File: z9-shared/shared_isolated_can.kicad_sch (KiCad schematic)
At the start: 6 parts, among them U951 ISO1042-Q1

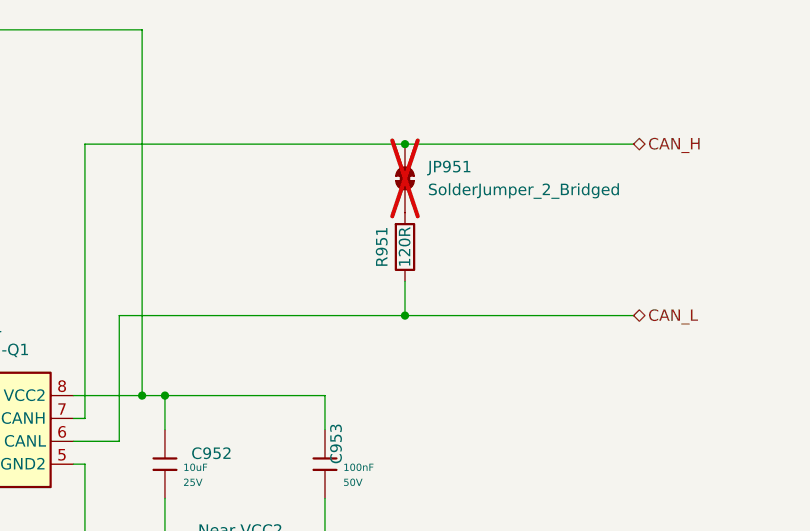
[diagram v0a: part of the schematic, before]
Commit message: lcsc components and cleanup
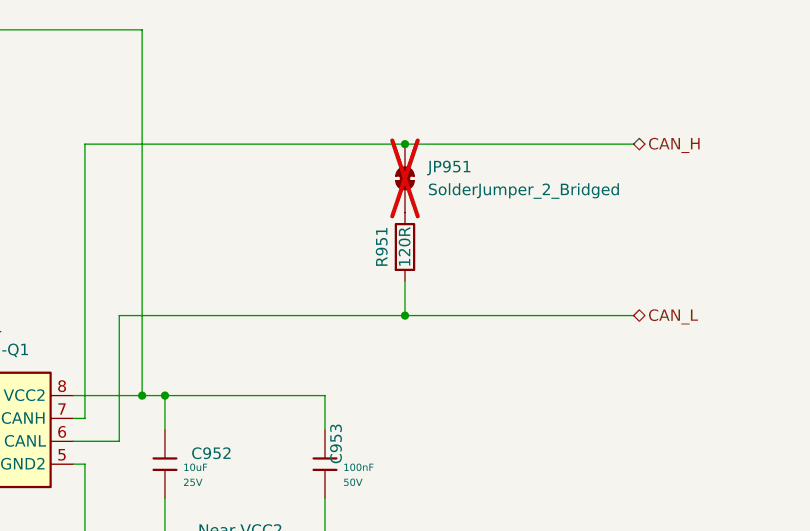
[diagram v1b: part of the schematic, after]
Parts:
- R951: footprint Resistor_SMD:R_0805_2012Metric -> dnt:R_1206_3216Metric; symbol dnt_global:Resisitor_120R_0805 -> dnt_global:Resistor_-_1206,120Ω; Attrition Qty (none) -> 10; Category (none) -> Resistors,Chip Resistor - Surface Mount; Class (none) -> Basic Component; LCSC (none) -> C17909; Manufacturer (none) -> UNI-ROYAL(Uniroyal Elec); Minimum Qty (none) -> 15; Operating Temperature Range (none) -> -55°C~+155°C; Overload Voltage (Max) (none) -> 200V; Part (none) -> 1206W4F1200T5E; Power(Watts) (none) -> 250mW; Price (none) -> 0.007USD; Process (none) -> SMT; Resistance (none) -> 120Ω; Stock (none) -> 622568; Temperature Coefficient (none) -> ±100ppm/°C; Tolerance (none) -> ±1%; Type (none) -> Thick Film Resistors
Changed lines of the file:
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@@
 	)
 	(symbol
-		(lib_id "dnt_global:Resisitor_120R_0805")
+		(lib_id "dnt_global:Resistor_-_1206,120Ω")
 		(at 193.04 73.66 0)
 		(mirror x)
@@
 			)
 		)
-		(property "Footprint" "Resistor_SMD:R_0805_2012Metric"
+		(property "Footprint" "dnt:R_1206_3216Metric"
 			(at 191.262 73.66 90)
 			(effects
@@
 			)
 		)
-		(property "Datasheet" "~"
-			(at 193.04 73.66 0)
-			(effects
-				(font
-					(size 1.27 1.27)
-				)
-				(hide yes)
-			)
-		)
-		(property "Description" "Resistor"
+		(property "Datasheet" "https://www.lcsc.com/datasheet/lcsc_datasheet_2206010145_UNI-ROYAL-Uniroyal-Elec-1206W4F1200T5E_C17909.pdf"
+			(at 193.04 73.66 0)
+			(effects
+				(font
+					(size 1.27 1.27)
+				)
+				(hide yes)
+			)
+		)
+		(property "Description" "250mW Thick Film Resistors 200V ±100ppm/°C ±1% 120Ω 1206 Chip Resistor - Surface Mount ROHS"
 			(at 193.04 73.66 0)
 			(effects
@@
 			(effects
 				(font
+					(size 1.27 1.27)
+				)
+				(hide yes)
+			)
+		)
+		(property "LCSC" "C17909"
+			(at 193.04 73.66 0)
+			(effects
+				(font
+					(size 1.27 1.27)
+				)
+				(hide yes)
+			)
+		)
+		(property "Stock" "622568"
+			(at 193.04 73.66 0)
+			(effects
+				(font
+					(size 1.27 1.27)
+				)
+				(hide yes)
+			)
+		)
+		(property "Price" "0.007USD"
+			(at 193.04 73.66 0)
+			(effects
+				(font
+					(size 1.27 1.27)
+				)
+				(hide yes)
+			)
+		)
+		(property "Process" "SMT"
+			(at 193.04 73.66 0)
+			(effects
+				(font
+					(size 1.27 1.27)
+				)
+				(hide yes)
+			)
+		)
+		(property "Minimum Qty" "15"
+			(at 193.04 73.66 0)
+			(effects
+				(font
+					(size 1.27 1.27)
+				)
+				(hide yes)
+			)
+		)
+		(property "Attrition Qty" "10"
+			(at 193.04 73.66 0)
+			(effects
+				(font
+					(size 1.27 1.27)
+				)
+				(hide yes)
+			)
+		)
+		(property "Class" "Basic Component"
+			(at 193.04 73.66 0)
+			(effects
+				(font
+					(size 1.27 1.27)
+				)
+				(hide yes)
+			)
+		)
+		(property "Category" "Resistors,Chip Resistor - Surface Mount"
+			(at 193.04 73.66 0)
+			(effects
+				(font
+					(size 1.27 1.27)
+				)
+				(hide yes)
+			)
+		)
+		(property "Manufacturer" "UNI-ROYAL(Uniroyal Elec)"
+			(at 193.04 73.66 0)
+			(effects
+				(font
+					(size 1.27 1.27)
+				)
+				(hide yes)
+			)
+		)
+		(property "Part" "1206W4F1200T5E"
+			(at 193.04 73.66 0)
+			(effects
+				(font
+					(size 1.27 1.27)
+				)
+				(hide yes)
+			)
+		)
+		(property "Resistance" "120Ω"
+			(at 193.04 73.66 0)
+			(effects
+				(font
+					(size 1.27 1.27)
+				)
+				(hide yes)
+			)
+		)
+		(property "Power(Watts)" "250mW"
+			(at 193.04 73.66 0)
+			(effects
+				(font
+					(size 1.27 1.27)
+				)
+				(hide yes)
+			)
+		)
+		(property "Type" "Thick Film Resistors"
+			(at 193.04 73.66 0)
+			(effects
+				(font
+					(size 1.27 1.27)
+				)
+				(hide yes)
+			)
+		)
+		(property "Overload Voltage (Max)" "200V"
+			(at 193.04 73.66 0)
+			(effects
+				(font
+					(size 1.27 1.27)
+				)
+				(hide yes)
+			)
+		)
+		(property "Operating Temperature Range" "-55°C~+155°C"
+			(at 193.04 73.66 0)
+			(effects
+				(font
+					(size 1.27 1.27)
+				)
+				(hide yes)
+			)
+		)
+		(property "Tolerance" "±1%"
+			(at 193.04 73.66 0)
+			(effects
+				(font
+					(size 1.27 1.27)
+				)
+				(hide yes)
+			)
+		)
+		(property "Temperature Coefficient" "±100ppm/°C"
+			(at 193.04 73.66 0)
+			(effects
+				(font

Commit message: fix 10uf 25v
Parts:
- C952: footprint PCM_JLCPCB:C_0603 -> dnt:C_0603_1608Metric; symbol PCM_JLCPCB-Capacitors:0603,10uF,(2) -> dnt_global:0603,10uF,_25V
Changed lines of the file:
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@@
 	)
 	(symbol
-		(lib_id "PCM_JLCPCB-Capacitors:0603,10uF,(2)")
+		(lib_id "dnt_global:0603,10uF,_25V")
 		(at 166.37 97.79 0)
 		(unit 1)
@@
 			)
 		)
-		(property "Footprint" "PCM_JLCPCB:C_0603"
+		(property "Footprint" "dnt:C_0603_1608Metric"
 			(at 164.592 97.79 90)
 			(effects
@@
 			(at 166.37 97.79 0)
 			(effects
-				(font
-					(size 1.27 1.27)
-				)
-				(hide yes)
-			)
-		)
-		(property "Order" ""
-			(at 166.37 97.79 0)
-			(effects
-				(font
-					(size 1.27 1.27)
-				)
-				(hide yes)
-			)
-		)
-		(property "PN" ""
-			(at 166.37 97.79 0)
-			(effects
-				(font
-					(size 1.27 1.27)
-				)
-				(hide yes)
-			)
-		)
-		(property "Part Number" ""
-			(at 166.37 97.79 0)
-			(effects
-				(font
-					(size 1.27 1.27)
-				)
-				(hide yes)
-			)
-		)
-		(property "Part#" ""
-			(at 166.37 97.79 0)
-			(effects
-				(font
-					(size 1.27 1.27)
-				)
-				(hide yes)
-			)
-		)
-		(property "Vendor" ""
-			(at 166.37 97.79 0)
-			(effects
-				(font
-					(size 1.27 1.27)
-				)
-				(hide yes)
-			)
-		)
-		(property "Voltage" ""
-			(at 166.37 97.79 0)
-			(effects

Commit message: continue lssc fixups
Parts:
- C951, C953: footprint PCM_JLCPCB:C_0603 -> dnt:C_0603_1608Metric; symbol PCM_JLCPCB-Capacitors:0603,100nF -> dnt_global:0603,100nF
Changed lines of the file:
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@@
 	)
 	(symbol
-		(lib_id "PCM_JLCPCB-Capacitors:0603,100nF")
+		(lib_id "dnt_global:0603,100nF")
 		(at 184.15 97.79 0)
 		(unit 1)
@@
 			)
 		)
-		(property "Footprint" "PCM_JLCPCB:C_0603"
+		(property "Footprint" "dnt:C_0603_1608Metric"
 			(at 182.372 97.79 90)
 			(effects
@@
 		(property "Temperature Coefficient" "X7R"
 			(at 184.15 97.79 0)
-			(effects
-				(font
-					(size 1.27 1.27)
-				)
-				(hide yes)
-			)
-		)
-		(property "Order" ""
-			(at 184.15 97.79 90)
-			(effects
-				(font
-					(size 1.27 1.27)
-				)
-				(hide yes)
-			)
-		)
-		(property "PN" ""
-			(at 184.15 97.79 90)
-			(effects
-				(font
-					(size 1.27 1.27)
-				)
-				(hide yes)
-			)
-		)
-		(property "Part Number" ""
-			(at 184.15 97.79 90)
-			(effects
-				(font
-					(size 1.27 1.27)
-				)
-				(hide yes)
-			)
-		)
-		(property "Part#" ""
-			(at 184.15 97.79 90)
-			(effects
-				(font
-					(size 1.27 1.27)
-				)
-				(hide yes)
-			)
-		)
-		(property "Vendor" ""
-			(at 184.15 97.79 90)
-			(effects
-				(font
-					(size 1.27 1.27)
-				)
-				(hide yes)
-			)
-		)
-		(property "Voltage" ""
-			(at 184.15 97.79 90)
 			(effects
 				(font
@@
 	)
 	(symbol
-		(lib_id "PCM_JLCPCB-Capacitors:0603,100nF")
+		(lib_id "dnt_global:0603,100nF")
 		(at 128.27 81.28 0)
 		(unit 1)
@@
 			)
 		)
-		(property "Footprint" "PCM_JLCPCB:C_0603"
+		(property "Footprint" "dnt:C_0603_1608Metric"
 			(at 126.492 81.28 90)
 			(effects
@@
 			(effects
 				(font
-					(size 1.27 1.27)
-				)
-				(hide yes)
-			)
-		)
-		(property "Order" ""
-			(at 128.27 81.28 90)
-			(effects
-				(font
-					(size 1.27 1.27)
-				)
-				(hide yes)
-			)
-		)
-		(property "PN" ""
-			(at 128.27 81.28 90)
-			(effects
-				(font
-					(size 1.27 1.27)
-				)
-				(hide yes)
-			)
-		)
-		(property "Part Number" ""
-			(at 128.27 81.28 90)
-			(effects
-				(font
-					(size 1.27 1.27)
-				)
-				(hide yes)
-			)
-		)
-		(property "Part#" ""
-			(at 128.27 81.28 90)
-			(effects
-				(font
-					(size 1.27 1.27)
-				)
-				(hide yes)
-			)
-		)
-		(property "Vendor" ""
-			(at 128.27 81.28 90)
-			(effects
-				(font
-					(size 1.27 1.27)
-				)
-				(hide yes)
-			)
-		)
-		(property "Voltage" ""
-			(at 128.27 81.28 90)
-			(effects
-				(font

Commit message: more change - generarte jlc
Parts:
- U951: JLCPCB Rotation Offset 90 -> 0
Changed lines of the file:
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@@
 			)
 		)
-		(property "JLCPCB Rotation Offset" "90"
+		(property "JLCPCB Rotation Offset" "0"
 			(at 120.65 85.852 0)
 			(effects

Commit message: more moving offset to library - tedious
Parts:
- U951: FT Rotation Offset (none) -> 90; JLCPCB Rotation Offset 0 -> (none)
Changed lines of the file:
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@@
 			)
 		)
-		(property "JLCPCB Rotation Offset" "0"
+		(property "FT Rotation Offset" "90"
 			(at 120.65 85.852 0)
 			(effects
 				(font
-					(size 1.27 1.27)
-				)
-				(hide yes)
-			)
-		)
-		(property "Sim.Device" ""
-			(at 146.05 92.71 0)
-			(effects
-				(font
-					(size 1.27 1.27)
-				)
-				(hide yes)
-			)
-		)
-		(property "Sim.Pins" ""
-			(at 146.05 92.71 0)
-			(effects
-				(font
-					(size 1.27 1.27)
-				)
-				(hide yes)
-			)
-		)
-		(property "Silkscreen" ""
-			(at 146.05 92.71 0)
-			(effects
-				(font
-					(size 1.27 1.27)
-				)
-				(hide yes)
-			)
-		)
-		(property "Order" ""
-			(at 146.05 92.71 0)
-			(effects
-				(font
-					(size 1.27 1.27)
-				)
-				(hide yes)
-			)
-		)
-		(property "PN" ""
-			(at 146.05 92.71 0)
-			(effects
-				(font
-					(size 1.27 1.27)
-				)
-				(hide yes)
-			)
-		)
-		(property "Part Number" ""
-			(at 146.05 92.71 0)
-			(effects
-				(font
-					(size 1.27 1.27)
-				)
-				(hide yes)
-			)
-		)
-		(property "Part#" ""
-			(at 146.05 92.71 0)
-			(effects
-				(font
-					(size 1.27 1.27)
-				)
-				(hide yes)
-			)
-		)
-		(property "Vendor" ""
-			(at 146.05 92.71 0)
-			(effects
-				(font
-					(size 1.27 1.27)
-				)
-				(hide yes)
-			)
-		)
-		(property "Voltage" ""
-			(at 146.05 92.71 0)
-			(effects
-				(font
